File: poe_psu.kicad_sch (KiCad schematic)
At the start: 41 parts, among them T1 HR051142, U2 SI3404-A-GM, U3 EL3H7-G, U4 AN431

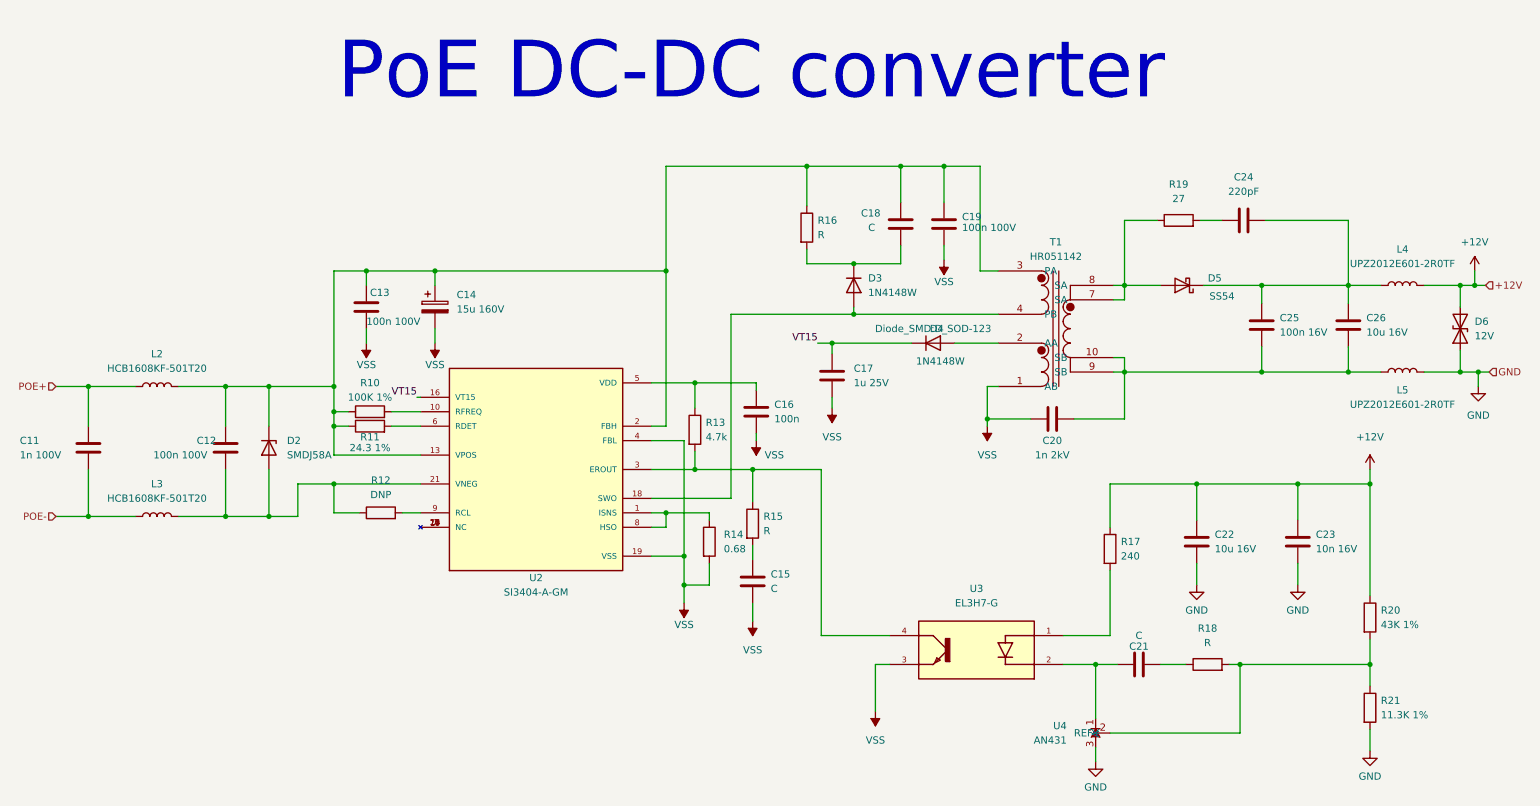
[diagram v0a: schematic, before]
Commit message: Update kicad files
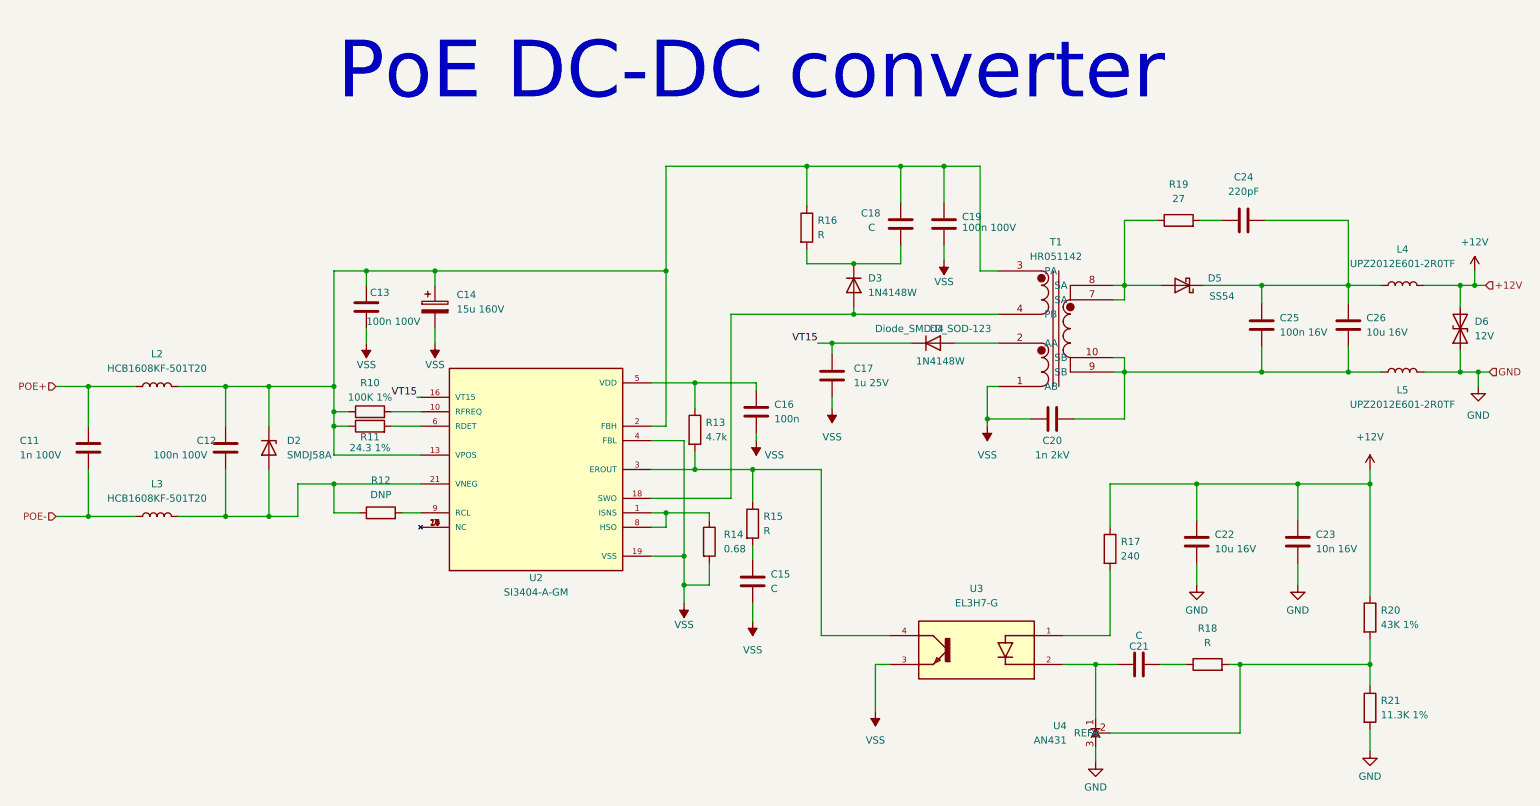
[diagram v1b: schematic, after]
